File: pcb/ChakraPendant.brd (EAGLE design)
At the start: 25.4 x 25.4 mm, 19 parts, among them Q1 MOSFET-NCHANNEL2N7002PW

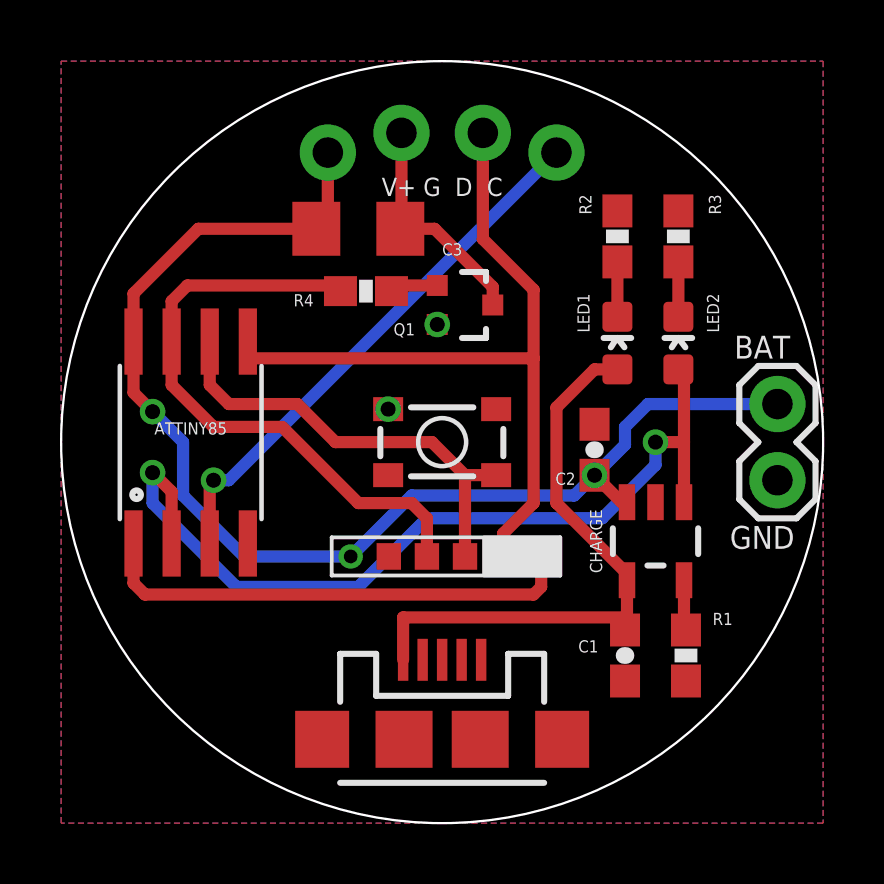
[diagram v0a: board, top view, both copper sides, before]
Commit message: WHO THE HELL KNOWS?
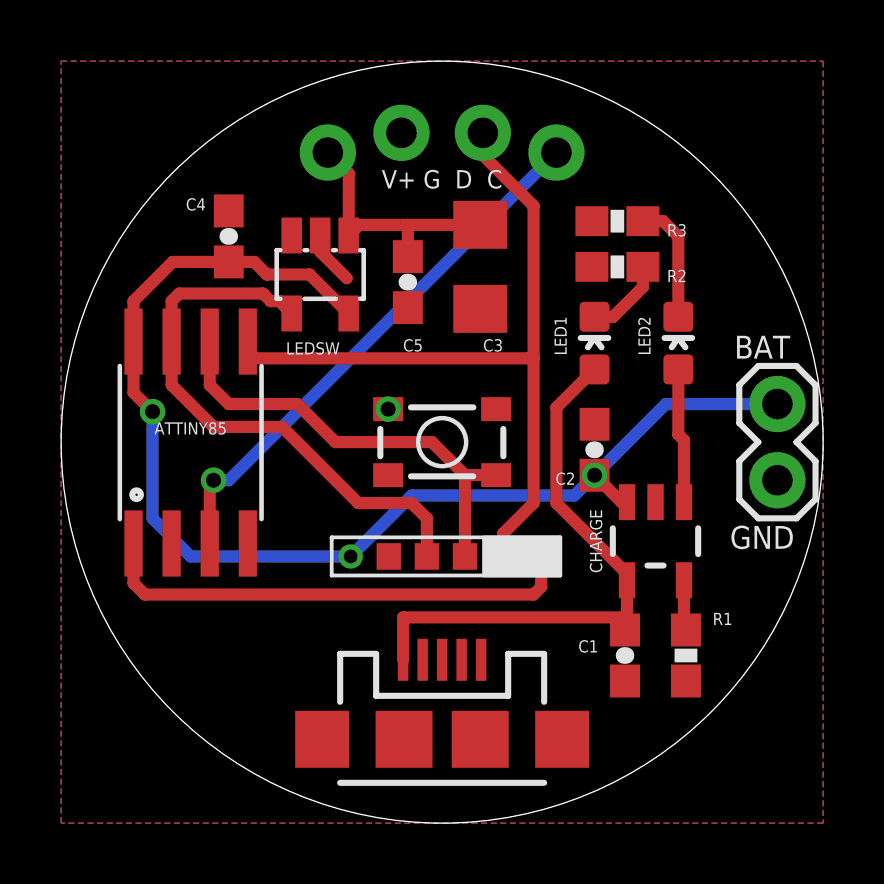
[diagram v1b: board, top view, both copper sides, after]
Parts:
- removed Q1: MOSFET-NCHANNEL2N7002PW, SparkFun-DiscreteSemi:SOT323
- removed R4: 220, SparkFun-Passives:0603-RES
- added C4: 1uF, SparkFun-Passives:0603-CAP
- added C5: 0.1uF, SparkFun-Passives:0603-CAP
- added LEDSW: (no value), IC:SOT23-5
- moved C3 4.26 mm to (14.0, 18.5), turned to 270 degrees
- moved R3 2.09 mm to (18.5, 20.1), turned to 0 degrees
- moved R2 1.02 mm to (18.5, 18.5), turned to 0 degrees
- moved LED1 0.76 mm to (17.8, 16.0)
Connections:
- removed net N$1: Q1.1, R4.2
- removed net N$2: C3.2, LEDPWR.2, Q1.3
- new net N$6: C3.1, C5.1, LEDPWR.1, LEDSW.1
- new net STAT: CHARGE.1, LED2.A
- net +4.1V: now also C4.1, LEDSW.5; no longer C3.1, LEDPWR.1
- net GND: now also C3.2, C4.2, C5.2, LEDPWR.2, LEDSW.2; no longer Q1.2
- net PB2-SCK: now also LEDSW.4; no longer R4.1
- net PB3-ADC3: no longer CHARGE.1, LED2.A
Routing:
- net PB3-ADC3: track 29.6 -> 0.00 mm, vias 2 -> 0
- net N$6: track 0.00 -> 8.64 mm
- net N$2: track 7.70 -> 0.00 mm
- net STAT: track 0.00 -> 4.50 mm
- net N$5: track 1.83 -> 4.07 mm
- net GND: track 0.00 -> 1.80 mm, vias 2 -> 1
- net N$1: track 1.60 -> 0.00 mm
- net PB2-SCK: track 20.3 -> 18.8 mm
- net N$4: track 1.83 -> 2.70 mm
- net +4.1V: track 41.7 -> 40.8 mm
- net USB5V: track 20.2 -> 19.4 mm
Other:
- board text added: "v5 Feb 7 2015"
- board text removed: "/Users/alex/Projects/BeautifulPixel/Logo/Logo Line.bmp"
- board text removed: "v5 Jan 21 2015"
